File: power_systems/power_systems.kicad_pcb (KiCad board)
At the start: 2 copper layers, 70 x 100 mm, 61 parts, among them J1 Screw_Terminal_01x02, J15 USB_B_Micro, J2 Screw_Terminal_01x02, J3 Screw_Terminal_01x02, J4 Conn_01x02_Pin, J5 Conn_01x02_Pin, J6 Conn_01x02_Pin, Q3 BSC520N15NS3GATMA1, Q4 BSC520N15NS3GATMA1, Q5 BSC520N15NS3GATMA1, U1 LTC7801EFE-PBF, U11 OPA333xxD, U12 OPA333xxD, U13 OPA333xxD, U2 TK25S06N1L_LQ, U4 LM5050MK-1/NOPB, U5 TK25S06N1L_LQ, U8 AMS1117-3.3, U9 LM5050MK-1/NOPB

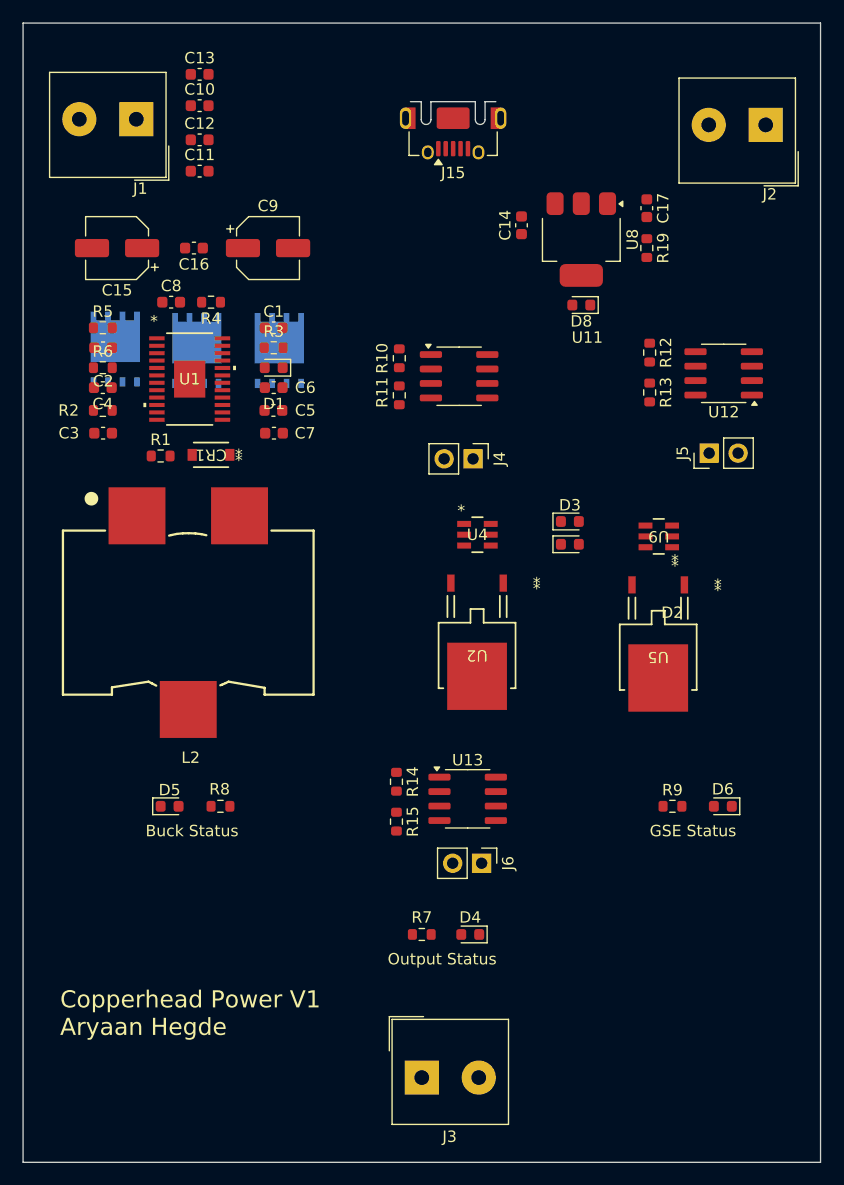
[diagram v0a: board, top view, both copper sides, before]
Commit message: Power systems routing v1
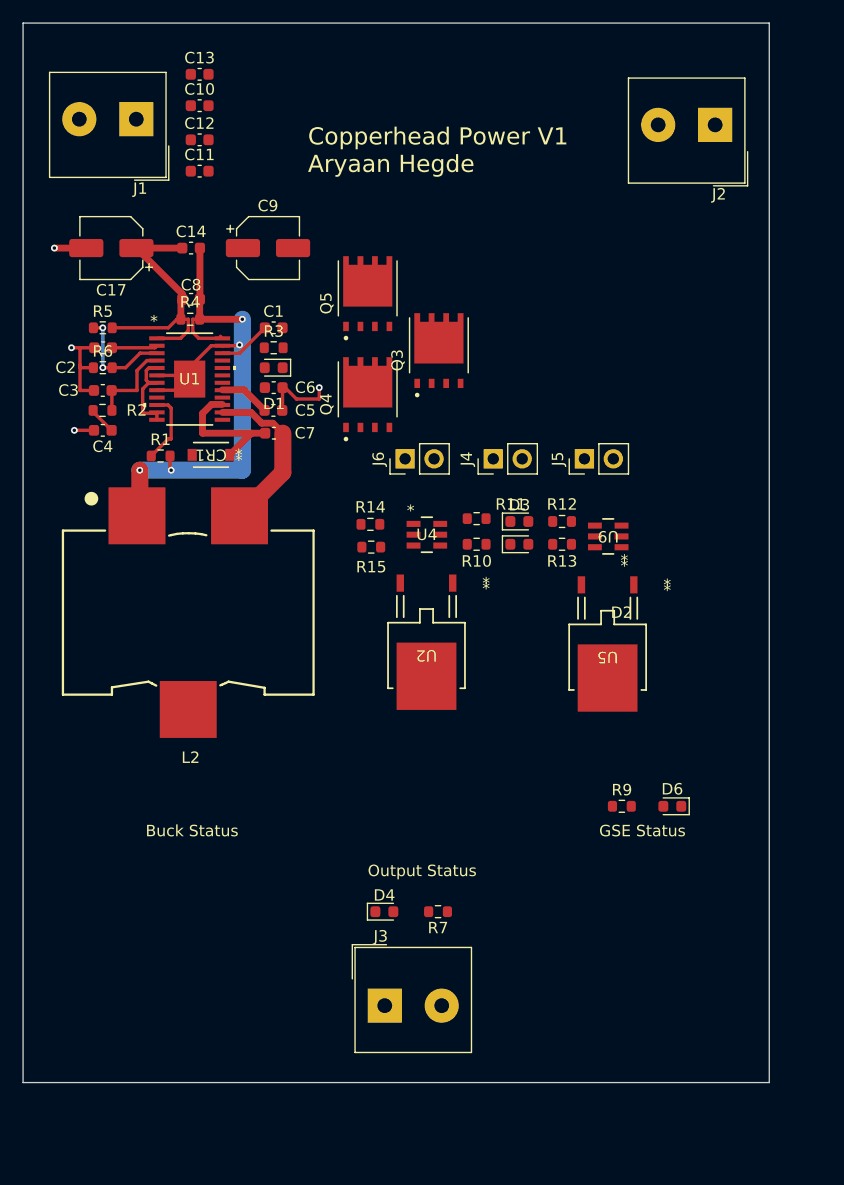
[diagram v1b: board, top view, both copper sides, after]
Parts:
- removed C15: 68uF, Capacitor_SMD:CP_Elec_5x3
- removed C16: 10uF, Capacitor_SMD:C_0603_1608Metric
- removed D5: LED_24, Diode_SMD:D_0603_1608Metric
- removed D8: LED_STM, Diode_SMD:D_0603_1608Metric
- removed J15: USB_B_Micro, Connector_USB:USB_Micro-AB_Molex_47590-0001
- removed R19: 1k5, Resistor_SMD:R_0603_1608Metric
- removed R8: 10k, Resistor_SMD:R_0603_1608Metric
- removed U11, U12, U13: OPA333xxD, Package_SO:SOIC-8_3.9x4.9mm_P1.27mm
- removed U8: AMS1117-3.3, Package_TO_SOT_SMD:SOT-223-3_TabPin2
- C14: value 22uF -> 10uF
- C17: value 22uF -> 68uF; footprint Capacitor_SMD:C_0603_1608Metric -> Capacitor_SMD:CP_Elec_5x3
- Q3, Q4, Q5: moved to F.Cu
- moved C17 47.1 mm to (107.8, 63.2), turned to 180 degrees
- moved J6 36.1 mm to (133.5, 81.8), turned to 90 degrees
- moved C14 29.1 mm to (114.8, 63.2), turned to 0 degrees
- moved Q3 28.4 mm to (136.5, 72.2)
- moved R15 24.2 mm to (130.6, 89.5), turned to 0 degrees
- moved R14 22.7 mm to (130.5, 87.5), turned to 180 degrees
- moved R10 17.7 mm to (139.8, 89.2), turned to 180 degrees
- moved R12 16.7 mm to (147.3, 87.2), turned to 180 degrees
- moved Q5 15.8 mm to (130.2, 67.2)
- moved R13 15.4 mm to (147.3, 89.2), turned to 0 degrees
- moved R11 12.8 mm to (139.8, 87.0), turned to 0 degrees
- moved J5 11.0 mm to (149.3, 81.8)
- moved Q4 8.66 mm to (130.2, 76.1)
- moved D4 7.80 mm to (131.7, 121.5), turned to 0 degrees
- moved J3 7.10 mm to (131.8, 129.8)
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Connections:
- net +BATT renamed /battery_step_down/+BATT
- net +GSE renamed /input_power_terminals/+GSE
- net +VOUT renamed /output_power_terminals/+VOUT
- C14 pad 1: GND -> /battery_step_down/SENSE-
- C14 pad 2: +VBUS -> GND
- C17 pad 1: GND -> /battery_step_down/SENSE-
- C17 pad 2: +3.3V -> GND
- C8 pad 1: /battery_step_down/SENSE+ -> GND
- D2 pad 1: +VBUCK -> /battery_step_down/SENSE-
- J4 pad 1: /sense_terminals/VBUCK_SENSE -> /output_power_terminals/VBUCK_SENSE
- J5 pad 1: /sense_terminals/GSE_SENSE -> /output_power_terminals/GSE_SENSE
- J6 pad 1: /sense_terminals/VOUT_SENSE -> /output_power_terminals/VOUT_SENSE
- L2 pad 2: /battery_step_down/SENSE+ -> GND
- R10 pad 1: +VBUCK -> /battery_step_down/SENSE-
- R10 pad 2: Net-(U11-+) -> /output_power_terminals/VBUCK_SENSE
- R11 pad 1: Net-(U11-+) -> /output_power_terminals/VBUCK_SENSE
- R12 pad 2: Net-(U12-+) -> /output_power_terminals/GSE_SENSE
- R13 pad 1: Net-(U12-+) -> /output_power_terminals/GSE_SENSE
- R14 pad 2: Net-(U13-+) -> /output_power_terminals/VOUT_SENSE
- R15 pad 1: Net-(U13-+) -> /output_power_terminals/VOUT_SENSE
- R3 pad 1: +VBUCK -> /battery_step_down/SENSE-
- R4 pad 1: /battery_step_down/SENSE+ -> GND
- R5 pad 1: Net-(U1-VFB) -> GND
- R6 pad 2: Net-(U1-VFB) -> GND
- U1 pad 24: /battery_step_down/SENSE+ -> GND
- U1 pad 3: Net-(U1-VFB) -> GND
- U1 pad 9: /battery_step_down/POWER_GOOD -> unconnected-(U1-PGOOD-Pad9)
- U2 pad 3: +VBUCK -> /battery_step_down/SENSE-
- U4 pad 4: +VBUCK -> /battery_step_down/SENSE-
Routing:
- net GND: track 0.00 -> 83.9 mm, vias 0 -> 10
- net /battery_step_down/SENSE-: track 0.00 -> 23.0 mm
- net /battery_step_down/SW: track 0.00 -> 14.9 mm
- net Net-(U1-CRUMPEN): track 0.00 -> 13.1 mm
- net Net-(U1-BOOST): track 0.00 -> 12.0 mm
- net Net-(U1-ITH): track 0.00 -> 7.84 mm
- net Net-(U1-FREQ): track 0.00 -> 6.44 mm
- net /battery_step_down/DRVCC: track 0.00 -> 4.45 mm
- net Net-(U1-SS): track 0.00 -> 4.02 mm
- net Net-(C4-Pad1): track 0.00 -> 2.42 mm
- added copper zone on In1.Cu, net GND
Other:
- board size 70 x 100 mm -> 65.5 x 93 mm
- copper layers 2 -> 4
